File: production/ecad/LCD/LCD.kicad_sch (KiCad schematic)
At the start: 1 part, among them J2 214721-0100

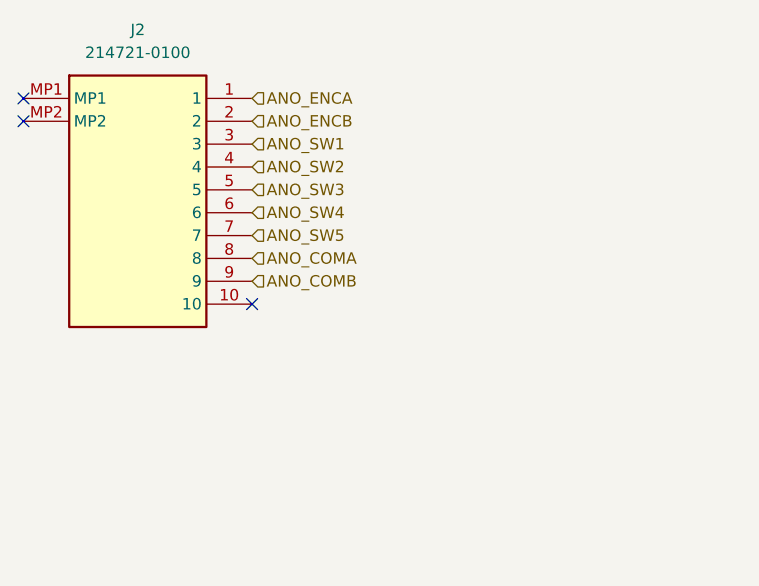
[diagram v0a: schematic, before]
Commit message: schematic draft merged w neha
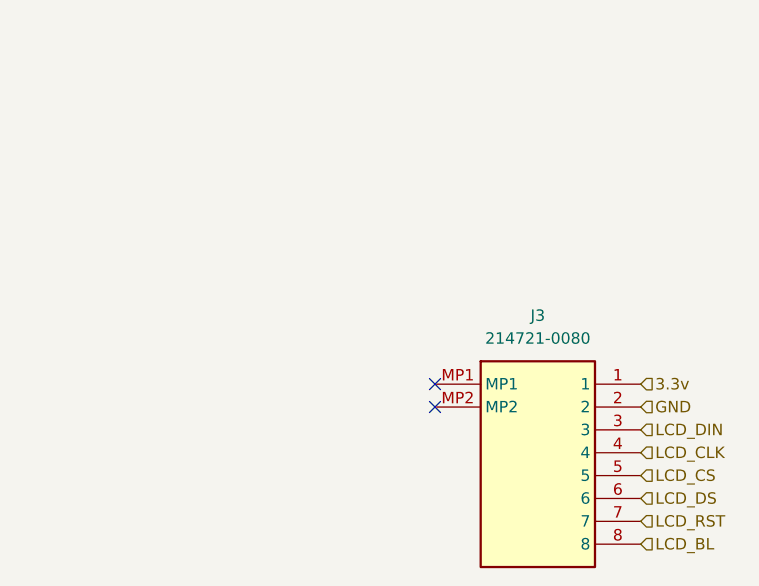
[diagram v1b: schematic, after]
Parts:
- removed J2: 214721-0100, 2147210100, symbol dialheader:214721-0100
- added J3: 214721-0080, 2147210080, symbol 8positionheader:214721-0080
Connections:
- new net 3.3v: J3.1
- new net GND: J3.2
- new net LCD_BL: J3.8
- new net LCD_CLK: J3.4
- new net LCD_CS: J3.5
- new net LCD_DIN: J3.3
- new net LCD_DS: J3.6
- new net LCD_RST: J3.7
- no-connect marks 3 -> 2
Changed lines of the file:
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@@
 	(paper "A4")
 	(no_connect
-		(at 119.38 91.44)
+		(at 139.7 102.87)
 	)
 	(no_connect
-		(at 93.98 68.58)
-	)
-	(no_connect
-		(at 93.98 71.12)
-	)
-	(hierarchical_label "ANO_SW1"
-		(shape input)
-		(at 119.38 73.66 0)
-		(fields_autoplaced yes)
-		(effects
-			(font
-				(size 1.27 1.27)
-			)
-			(justify left)
-		)
-	)
-	(hierarchical_label "ANO_COMB"
-		(shape input)
-		(at 119.38 88.9 0)
-		(fields_autoplaced yes)
-		(effects
-			(font
-				(size 1.27 1.27)
-			)
-			(justify left)
-		)
-	)
-	(hierarchical_label "ANO_ENCA"
-		(shape input)
-		(at 119.38 68.58 0)
-		(fields_autoplaced yes)
-		(effects
-			(font
-				(size 1.27 1.27)
-			)
-			(justify left)
-		)
-	)
-	(hierarchical_label "ANO_SW3"
-		(shape input)
-		(at 119.38 78.74 0)
-		(fields_autoplaced yes)
-		(effects
-			(font
-				(size 1.27 1.27)
-			)
-			(justify left)
-		)
-	)
-	(hierarchical_label "ANO_ENCB"
-		(shape input)
-		(at 119.38 71.12 0)
-		(fields_autoplaced yes)
-		(effects
-			(font
-				(size 1.27 1.27)
-			)
-			(justify left)
-		)
-	)
-	(hierarchical_label "ANO_SW2"
-		(shape input)
-		(at 119.38 76.2 0)
-		(fields_autoplaced yes)
-		(effects
-			(font
-				(size 1.27 1.27)
-			)
-			(justify left)
-		)
-	)
-	(hierarchical_label "ANO_SW5"
-		(shape input)
-		(at 119.38 83.82 0)
-		(fields_autoplaced yes)
-		(effects
-			(font
-				(size 1.27 1.27)
-			)
-			(justify left)
-		)
-	)
-	(hierarchical_label "ANO_COMA"
-		(shape input)
-		(at 119.38 86.36 0)
-		(fields_autoplaced yes)
-		(effects
-			(font
-				(size 1.27 1.27)
-			)
-			(justify left)
-		)
-	)
-	(hierarchical_label "ANO_SW4"
-		(shape input)
-		(at 119.38 81.28 0)
+		(at 139.7 100.33)
+	)
+	(hierarchical_label "LCD_CLK"
+		(shape input)
+		(at 162.56 107.95 0)
+		(fields_autoplaced yes)
+		(effects
+			(font
+				(size 1.27 1.27)
+			)
+			(justify left)
+		)
+	)
+	(hierarchical_label "LCD_DIN"
+		(shape input)
+		(at 162.56 105.41 0)
+		(fields_autoplaced yes)
+		(effects
+			(font
+				(size 1.27 1.27)
+			)
+			(justify left)
+		)
+	)
+	(hierarchical_label "LCD_RST"
+		(shape input)
+		(at 162.56 115.57 0)
+		(fields_autoplaced yes)
+		(effects
+			(font
+				(size 1.27 1.27)
+			)
+			(justify left)
+		)
+	)
+	(hierarchical_label "3.3v"
+		(shape input)
+		(at 162.56 100.33 0)
+		(fields_autoplaced yes)
+		(effects
+			(font
+				(size 1.27 1.27)
+			)
+			(justify left)
+		)
+	)
+	(hierarchical_label "LCD_CS"
+		(shape input)
+		(at 162.56 110.49 0)
+		(fields_autoplaced yes)
+		(effects
+			(font
+				(size 1.27 1.27)
+			)
+			(justify left)
+		)
+	)
+	(hierarchical_label "LCD_DS"
+		(shape input)
+		(at 162.56 113.03 0)
+		(fields_autoplaced yes)
+		(effects
+			(font
+				(size 1.27 1.27)
+			)
+			(justify left)
+		)
+	)
+	(hierarchical_label "GND"
+		(shape input)
+		(at 162.56 102.87 0)
+		(fields_autoplaced yes)
+		(effects
+			(font
+				(size 1.27 1.27)
+			)
+			(justify left)
+		)
+	)
+	(hierarchical_label "LCD_BL"
+		(shape input)
+		(at 162.56 118.11 0)
 		(fields_autoplaced yes)
 		(effects
@@
 	)
 	(symbol
-		(lib_id "dialheader:214721-0100")
-		(at 93.98 68.58 0)
+		(lib_id "8positionheader:214721-0080")
+		(at 139.7 100.33 0)
 		(unit 1)
 		(exclude_from_sim no)
@@
 		(dnp no)
 		(fields_autoplaced yes)
-		(property "Reference" "J2"
-			(at 106.68 60.96 0)
-			(effects
-				(font
-					(size 1.27 1.27)
-				)
-			)
-		)
-		(property "Value" "214721-0100"
-			(at 106.68 63.5 0)
-			(effects
-				(font
-					(size 1.27 1.27)
-				)
-			)
-		)
-		(property "Footprint" "2147210100"
-			(at 115.57 163.5 0)
-			(effects
-				(font
-					(size 1.27 1.27)
-				)
-				(justify left top)
-				(hide yes)
-			)
-		)
-		(property "Datasheet" "https://www.molex.com/pdm_docs/sd/2147210100_sd.pdf"
-			(at 115.57 263.5 0)
-			(effects
-				(font
-					(size 1.27 1.27)
-				)
-				(justify left top)
-				(hide yes)
-			)
-		)
-		(property "Description" "MOLEX - 214721-0100 - Pin Header, Signal, Wire-to-Board, 0.8 mm, 1 Rows, 10 Contacts, Surface Mount Right Angle"
-			(at 93.98 68.58 0)
+		(property "Reference" "J3"
+			(at 151.13 92.71 0)
+			(effects
+				(font
+					(size 1.27 1.27)
+				)
+			)
+		)
+		(property "Value" "214721-0080"
+			(at 151.13 95.25 0)
+			(effects
+				(font
+					(size 1.27 1.27)
+				)
+			)
+		)
+		(property "Footprint" "2147210080"
+			(at 158.75 195.25 0)
+			(effects
+				(font
+					(size 1.27 1.27)
+				)
+				(justify left top)
+				(hide yes)
+			)
+		)
+		(property "Datasheet" "https://www.molex.com/pdm_docs/sd/2147210080_sd.pdf"
+			(at 158.75 295.25 0)
+			(effects
+				(font
+					(size 1.27 1.27)
+				)
+				(justify left top)
+				(hide yes)
+			)
+		)
+		(property "Description" "Zero-Hachi Header, 0.80mm Pitch, Single Row, Right-Angle, Surface Mount, Matte Tin (Sn) Plating, Friction Lock, 8 Circuits, Tape and Reel"
+			(at 139.7 100.33 0)
 			(effects
 				(font
@@
 		)
 		(property "Height" "1.8"
-			(at 115.57 463.5 0)
-			(effects
-				(font
-					(size 1.27 1.27)
-				)
-				(justify left top)
-				(hide yes)
-			)
-		)
-		(property "Mouser Part Number" "538-214721-0100"
-			(at 115.57 563.5 0)
-			(effects
-				(font
-					(size 1.27 1.27)
-				)
-				(justify left top)
-				(hide yes)
-			)
-		)
-		(property "Mouser Price/Stock" "https://www.mouser.co.uk/ProductDetail/Molex/214721-0100?qs=MyNHzdoqoQJCc4Zxlj0GUQ%3D%3D"
-			(at 115.57 663.5 0)
+			(at 158.75 495.25 0)
+			(effects
+				(font
+					(size 1.27 1.27)
+				)
+				(justify left top)
+				(hide yes)
+			)
+		)
+		(property "Mouser Part Number" ""
+			(at 158.75 595.25 0)
+			(effects
+				(font
+					(size 1.27 1.27)
+				)
+				(justify left top)
+				(hide yes)
+			)
+		)
+		(property "Mouser Price/Stock" ""
+			(at 158.75 695.25 0)
 			(effects
 				(font
@@
 		)
 		(property "Manufacturer_Name" "Molex"
-			(at 115.57 763.5 0)
-			(effects
-				(font
-					(size 1.27 1.27)
-				)
-				(justify left top)
-				(hide yes)
-			)
-		)
-		(property "Manufacturer_Part_Number" "214721-0100"
-			(at 115.57 863.5 0)
-			(effects
-				(font
-					(size 1.27 1.27)
-				)
-				(justify left top)
-				(hide yes)
-			)
-		)
-		(pin "10"
+			(at 158.75 795.25 0)
+			(effects
+				(font
+					(size 1.27 1.27)
+				)
+				(justify left top)
+				(hide yes)
+			)
+		)
+		(property "Manufacturer_Part_Number" "214721-0080"
+			(at 158.75 895.25 0)
+			(effects
+				(font
+					(size 1.27 1.27)
+				)
+				(justify left top)
+				(hide yes)
+			)
+		)
+		(pin "7"
+		)
+		(pin "2"
+		)
+		(pin "MP1"
+		)
+		(pin "6"
 		)
 		(pin "3"
 		)
+		(pin "MP2"
+		)
+		(pin "8"
+		)
+		(pin "5"
+		)
+		(pin "1"
+		)
 		(pin "4"
 		)
-		(pin "MP2"
-		)
-		(pin "5"
-		)
-		(pin "2"
-		)
-		(pin "6"
-		)
-		(pin "8"
-		)
-		(pin "9"
-		)
-		(pin "MP1"
-		)
-		(pin "1"
-		)
-		(pin "7"
-		)
 		(instances
-			(project ""
-				(path "/a34d77bc-8f6a-417e-a206-3165e6c5c658/56db885d-6988-4ba3-9c6c-3dd30ffbc985"
-					(reference "J2")
+			(project "Main"
+				(path "/a34d77bc-8f6a-417e-a206-3165e6c5c658/6d945d10-bd0c-4453-b6e0-f783497d7a3f"
+					(reference "J3")
 					(unit 1)
 				)

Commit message: merged with main
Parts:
- J3: footprint 2147210080 -> footprints:8positionheader
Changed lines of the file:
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@@
 			)
 		)
-		(property "Footprint" "2147210080"
+		(property "Footprint" "footprints:8positionheader"
 			(at 158.75 195.25 0)
 			(effects
